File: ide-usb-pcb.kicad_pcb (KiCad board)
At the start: 2 copper layers, 28 parts, among them J1 Conn_02x20_Odd_Even, J2 STM32F4_Discovery_Header, U1 TXS0108EPW, U2 TXS0108EPW

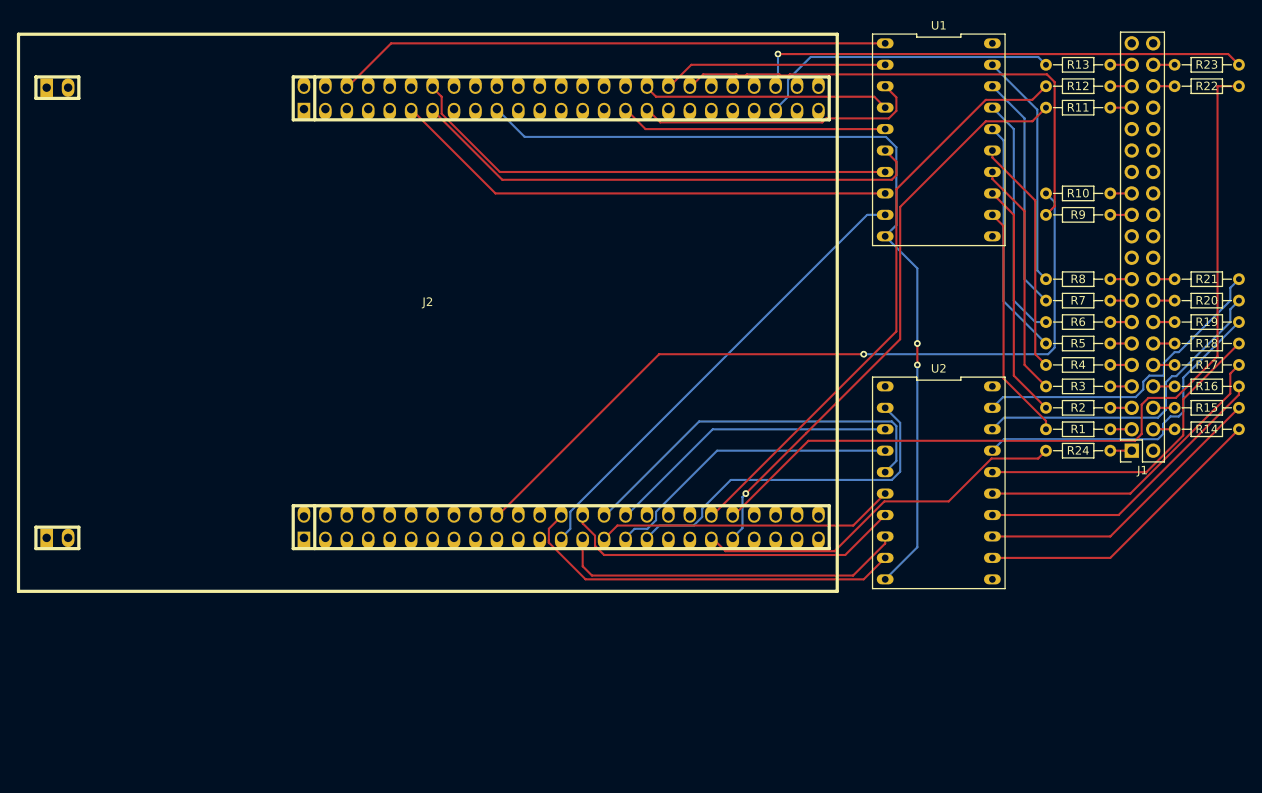
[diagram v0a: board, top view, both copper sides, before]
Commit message: New smaller and (maybe) cleaner PCB design
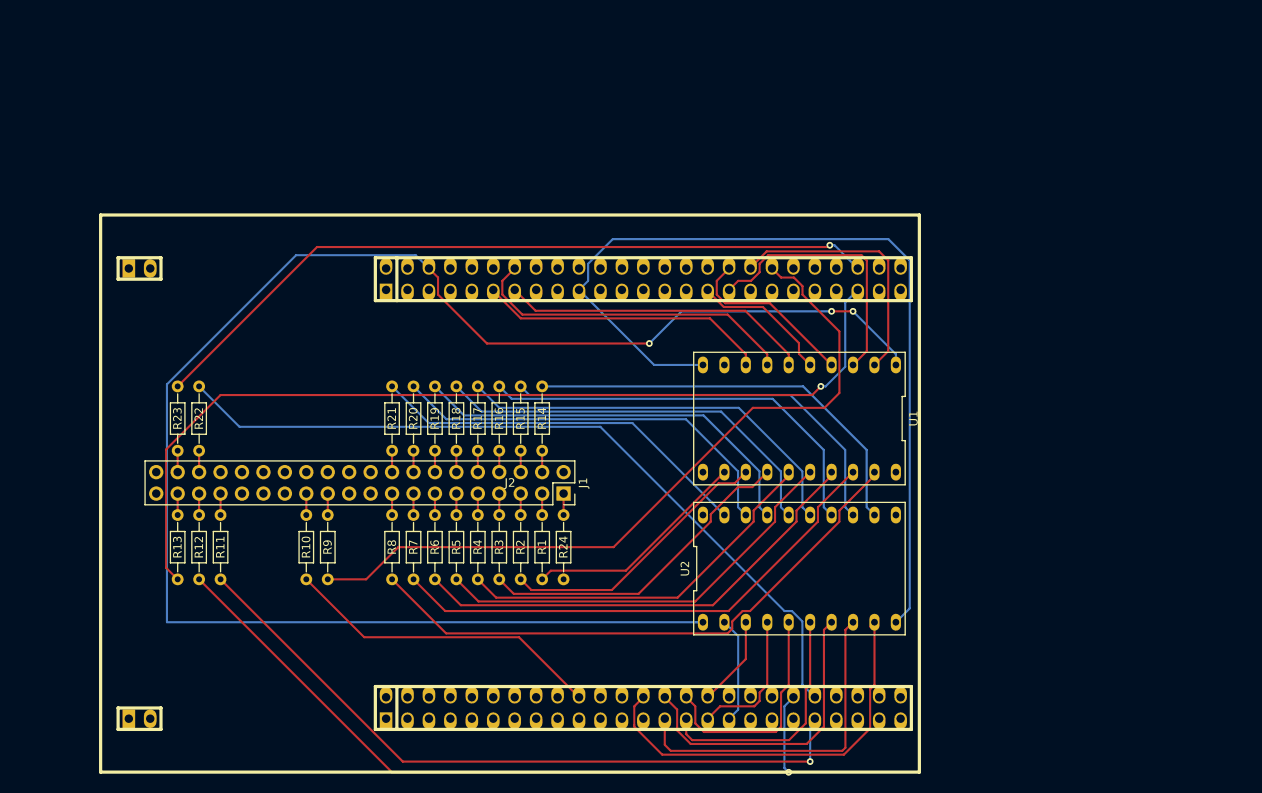
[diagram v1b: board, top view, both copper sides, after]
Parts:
- moved R23 131.4 mm to (45.7, 61.0), turned to 270 degrees
- moved R22 128.2 mm to (48.3, 61.0), turned to 270 degrees
- moved R13 122.7 mm to (45.7, 76.2), turned to 270 degrees
- moved R12 119.3 mm to (48.3, 76.2), turned to 270 degrees
- moved R11 115.9 mm to (50.8, 76.2), turned to 270 degrees
- moved R10 102.6 mm to (61.0, 76.2), turned to 270 degrees
- moved R21 101.1 mm to (71.1, 61.0), turned to 270 degrees
- moved R9 99.3 mm to (63.5, 76.2), turned to 270 degrees
- moved R20 98.3 mm to (73.7, 61.0), turned to 270 degrees
- moved R19 95.6 mm to (76.2, 61.0), turned to 270 degrees
- moved R18 92.8 mm to (78.7, 61.0), turned to 270 degrees
- moved R17 90.2 mm to (81.3, 61.0), turned to 270 degrees
- moved R8 89.6 mm to (71.1, 76.2), turned to 270 degrees
- moved R16 87.6 mm to (83.8, 61.0), turned to 270 degrees
- moved R7 86.4 mm to (73.7, 76.2), turned to 270 degrees
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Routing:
- net +3V3: track 66.0 -> 195.7 mm, vias 0 -> 3
- net /CS0: track 36.2 -> 110.2 mm, vias 0 -> 1
- net /DD7A: track 55.4 -> 0.00 mm
- net /DIOR: track 93.1 -> 38.1 mm, vias 1 -> 0
- net /RESET: track 45.2 -> 0.00 mm
- net /DD0B: track 28.0 -> 69.2 mm
- net /DD1B: track 28.0 -> 61.4 mm
- net /DD15A: track 42.1 -> 12.6 mm
- net /CS1: track 59.2 -> 88.5 mm
- net /DIOW: track 60.6 -> 88.7 mm
- net /DD2B: track 28.8 -> 55.8 mm
- net /DD6A: track 60.3 -> 34.4 mm
- net /DD4A: track 62.2 -> 36.9 mm
- net /DD14A: track 35.0 -> 10.8 mm
- net /DD3B: track 28.0 -> 50.3 mm
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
